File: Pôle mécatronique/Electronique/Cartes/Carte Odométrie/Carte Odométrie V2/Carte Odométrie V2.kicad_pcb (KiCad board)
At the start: 2 copper layers, 62.9 x 78.2 mm, 14 parts, among them J1 Conn_01x08, J2 Conn_01x05, J3 Conn_01x04, J4 Conn_01x07, J5 Conn_01x07, U1 TCAN332

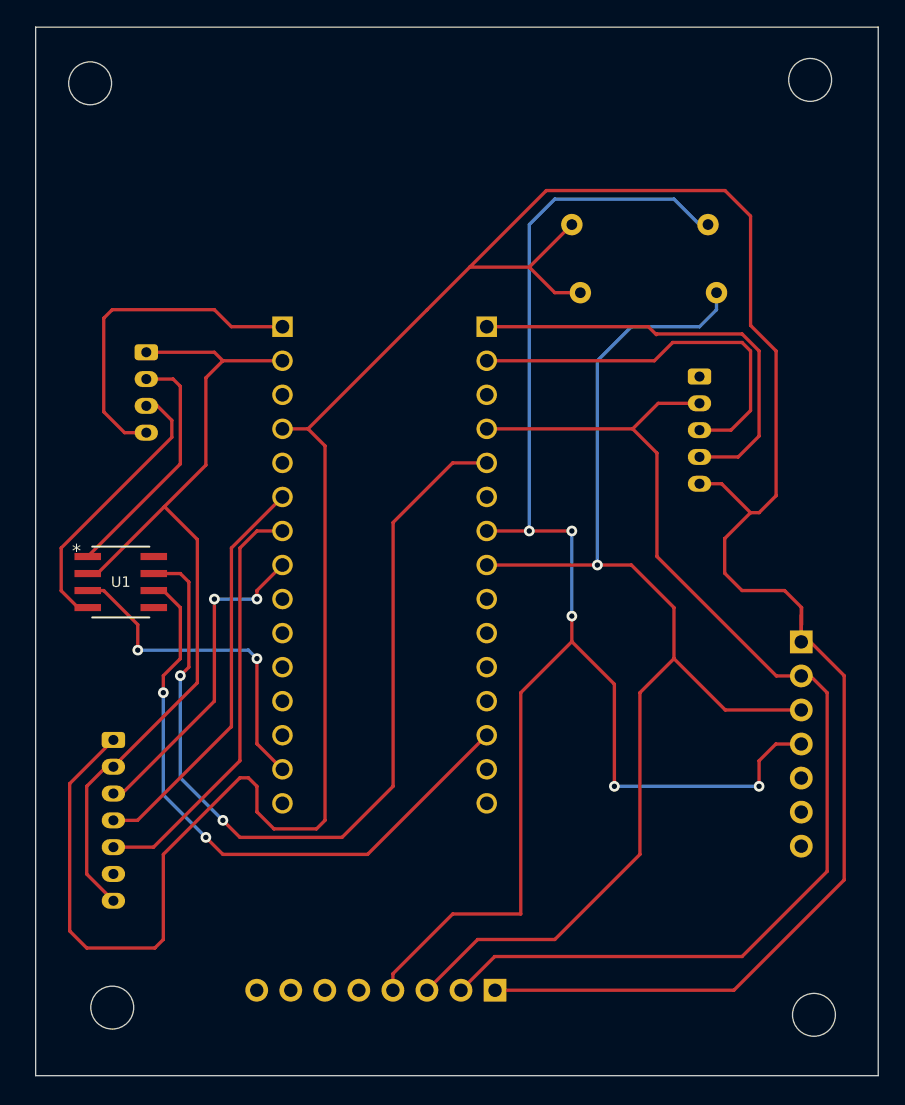
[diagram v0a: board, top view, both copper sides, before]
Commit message: Carte odométrie v2 "fini"
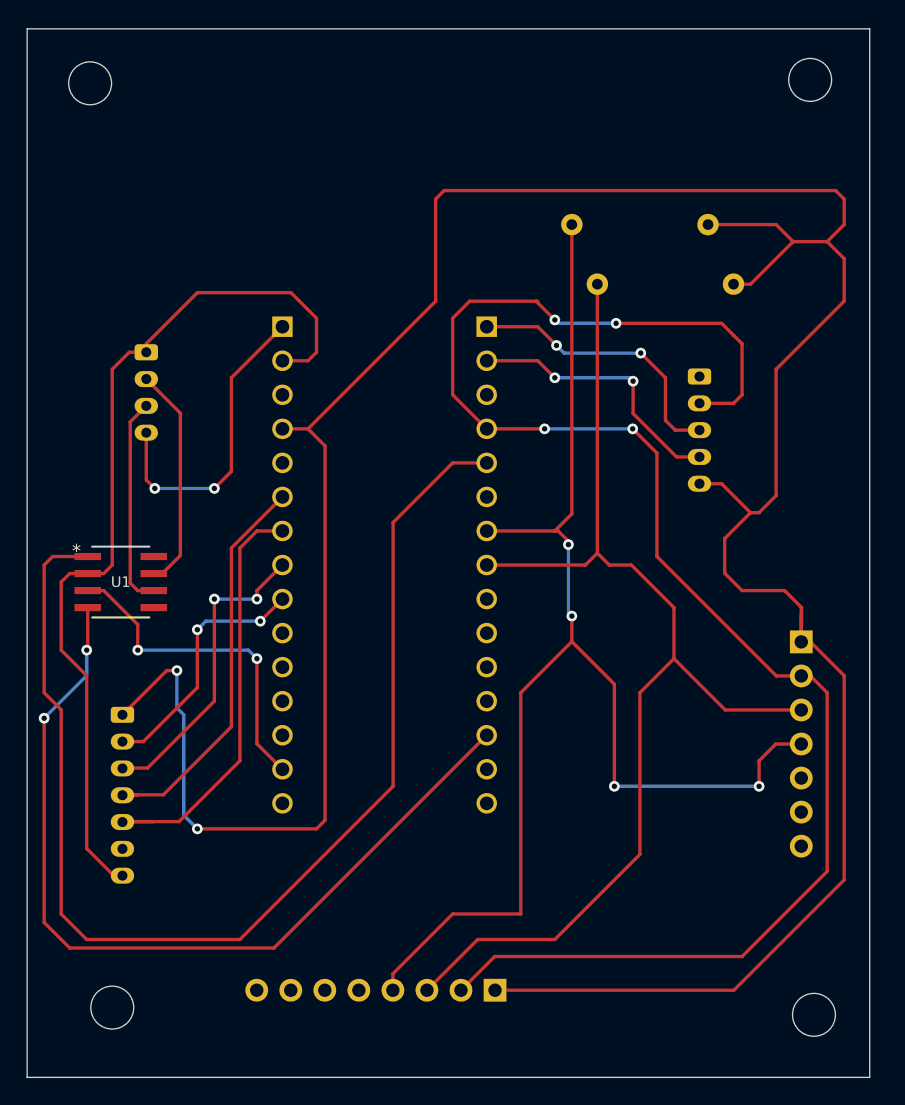
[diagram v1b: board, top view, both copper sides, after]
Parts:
- moved R1 10.2 mm to (174.0, 76.2), turned to 180 degrees
- moved R2 8.91 mm to (165.7, 80.6), turned to 0 degrees
- moved J4 1.99 mm to (130.3, 112.8)
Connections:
- A1 pad 3.13: CAN_L -> CAN_TX
- A1 pad 3.5: CAN_H -> CAN_RX
- A1 pad 4.9: unconnected-(A1-Pad4.9) -> SPI_CS
- J2 pad 3: UART1_RX -> UART1_TX
- J2 pad 4: UART1_TX -> UART1_RX
- J3 pad 2: CAN_RX -> CAN_H
- J3 pad 3: CAN_TX -> CAN_L
- J4 pad 2: GND -> SPI_CS
- J4 pad 6: unconnected-(J4-Pad6) -> (no net)
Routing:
- net CAN_RX: track 18.3 -> 88.9 mm
- net CAN_H: track 65.6 -> 16.8 mm, vias 2 -> 0
- net CAN_TX: track 21.0 -> 65.3 mm, vias 0 -> 2
- net GND: track 154.1 -> 189.7 mm, vias 0 -> 4
- net CAN_L: track 46.7 -> 15.7 mm, vias 2 -> 0
- net SPI_CS: track 0.00 -> 19.1 mm, vias 0 -> 2
- net I2C_SDA: track 115.6 -> 100.1 mm, vias 5 -> 4
- net UART1_TX: track 32.5 -> 21.2 mm, vias 0 -> 2
- net UART1_RX: track 29.4 -> 20.3 mm, vias 0 -> 2
- net I2C_SCL: track 92.9 -> 86.7 mm, vias 1 -> 0
- net +5V: track 228.5 -> 225.9 mm, vias 0 -> 2
- net +BATT: track 24.9 -> 23.0 mm, vias 0 -> 2
- net SPI_MISO: track 31.7 -> 33.3 mm
- net SPI_CLK: track 24.5 -> 23.8 mm
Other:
- board text added: "SPI_CS"
